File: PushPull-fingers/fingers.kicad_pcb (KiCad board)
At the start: 2 copper layers, 2 parts, among them P1 CONN_01X07, U1 fingerBoard

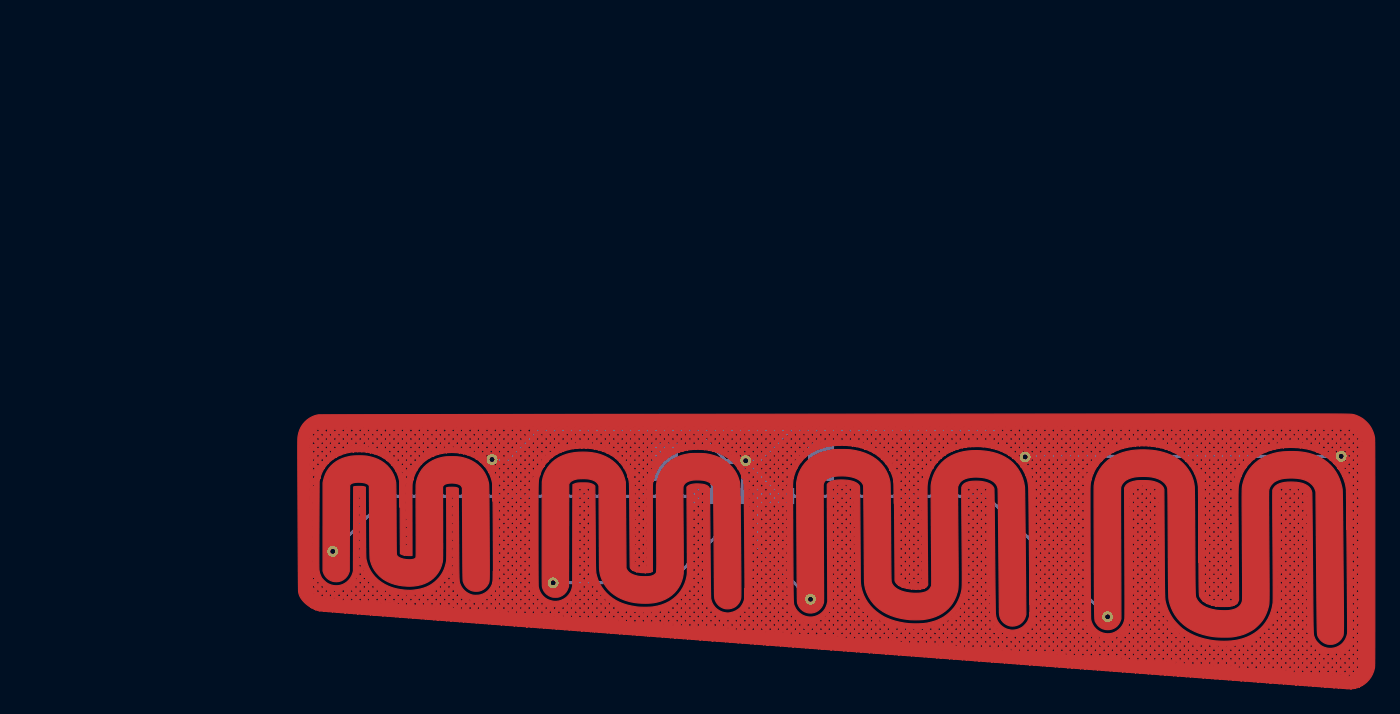
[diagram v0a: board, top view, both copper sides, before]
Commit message: production pcb kicad files and gerbers
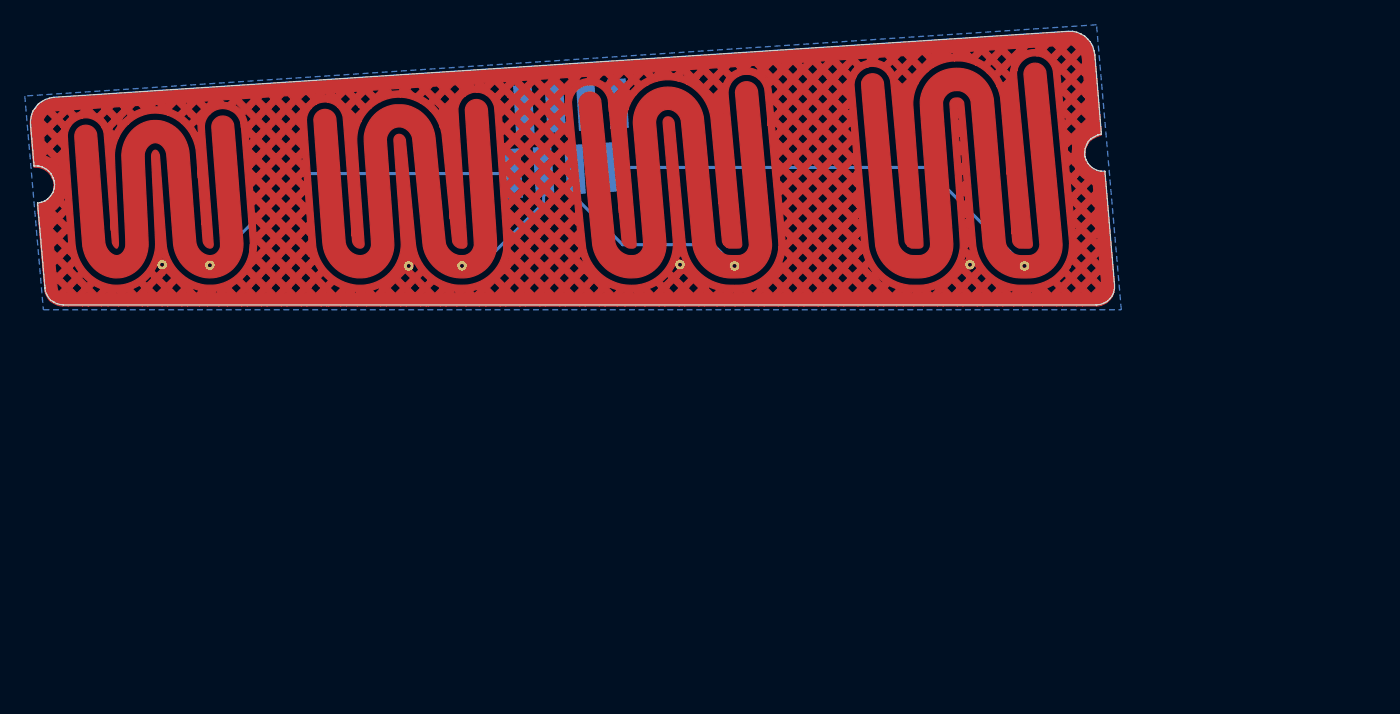
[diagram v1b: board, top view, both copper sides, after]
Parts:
- removed U1: fingerBoard, PushPull:pushPullFingersPad
- added P2: CONN_01X08, PushPull:PushPull_FingersPad, F.Cu at (127.2, 74.2)
- P1: value CONN_01X07 -> CapFingers; footprint Connectors_Molex:Connector_Molex_PicoBlade_53398-0771 -> PushPull:8_PIN_MM_conn
- moved P1 30.1 mm to (120.8, 75.5), turned to 3.7 degrees
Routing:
- net GND: track 92.5 -> 0.00 mm
- net Net-(P1-Pad5): track 10.1 -> 17.4 mm
- net Net-(P1-Pad7): track 29.7 -> 37.0 mm
- net Net-(P1-Pad3): track 18.3 -> 11.2 mm
- net Net-(P1-Pad1): track 31.2 -> 27.5 mm
- added copper zone on B.Cu, net GND
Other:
- board outline added: 87.5 x 22.1 mm
- rule pad_to_mask_clearance: 0 -> 0.2
